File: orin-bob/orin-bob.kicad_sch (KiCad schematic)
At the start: 0 parts

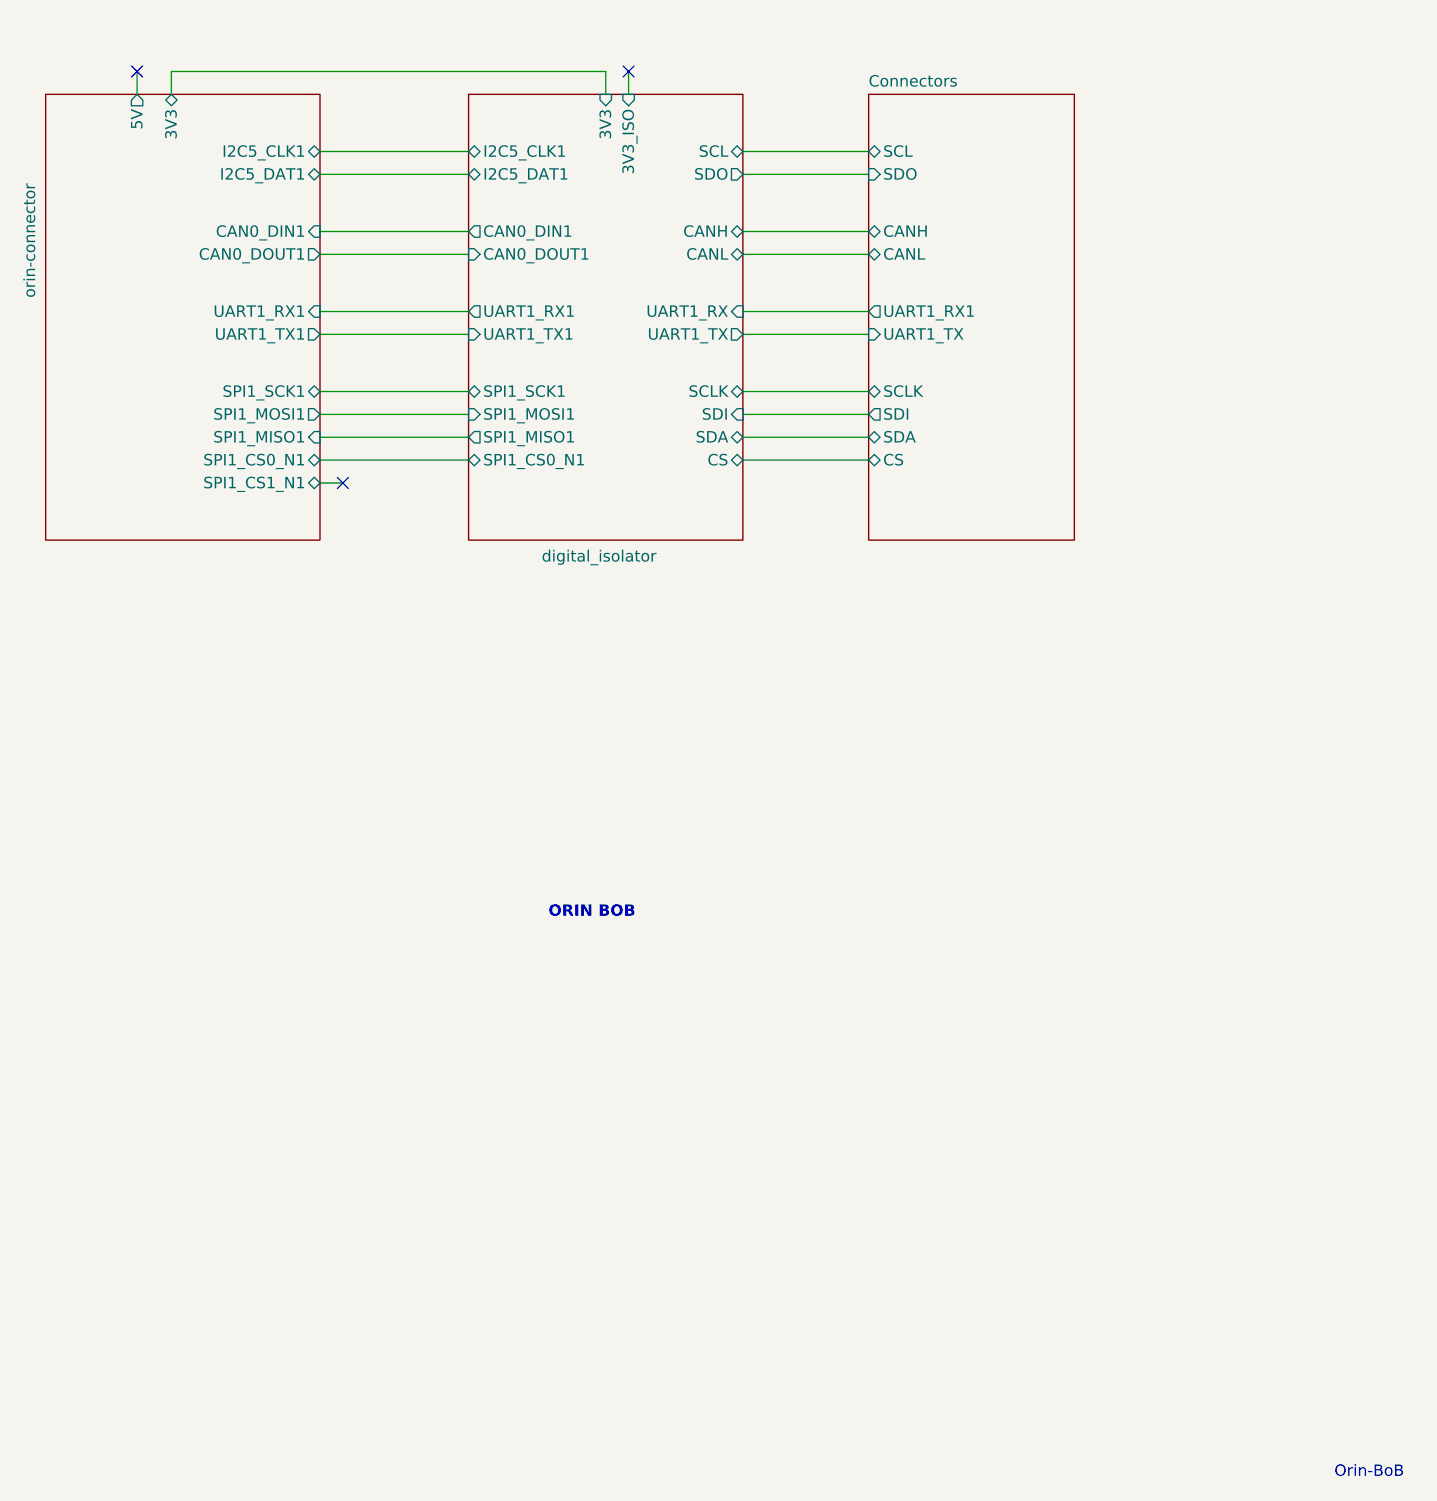
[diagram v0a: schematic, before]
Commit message: Updated bob pcb
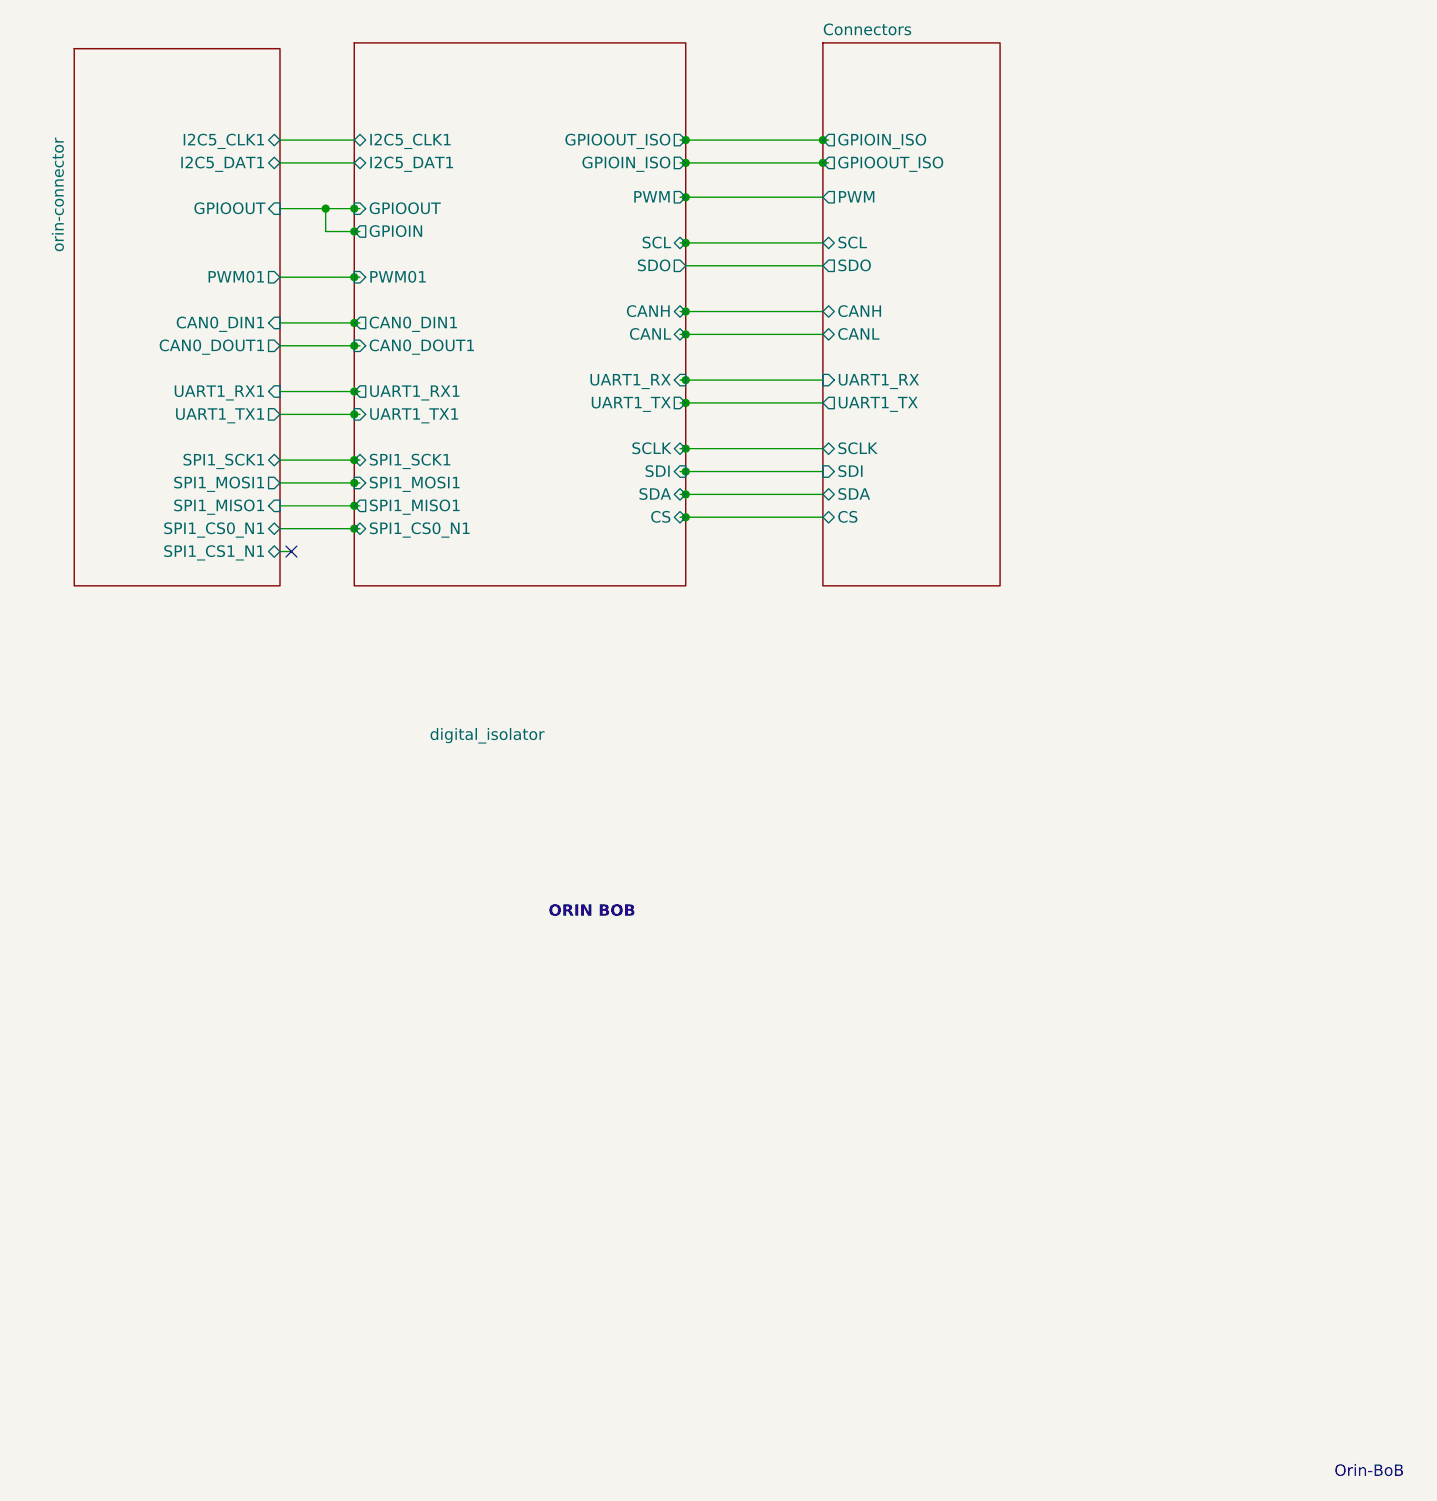
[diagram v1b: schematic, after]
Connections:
- no-connect marks 3 -> 1
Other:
- sheet Connectors ports: added GPIOIN_ISO, GPIOOUT_ISO, PWM, UART1_RX; removed UART1_RX1
- sheet digital_isolator ports: added GPIOIN, GPIOIN_ISO, GPIOOUT, GPIOOUT_ISO, PWM, PWM01; removed 3V3, 3V3_ISO
- sheet orin-connector ports: added GPIOOUT, PWM01; removed 3V3, 5V
